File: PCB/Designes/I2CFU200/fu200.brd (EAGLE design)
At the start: 100 x 80 mm, 19 parts, among them IC2 LM358N, T1 2N3565, T2 2N3565, T3 2N3565, U1 ATMEGA328P-AU, X1 250-111, X3 250-706

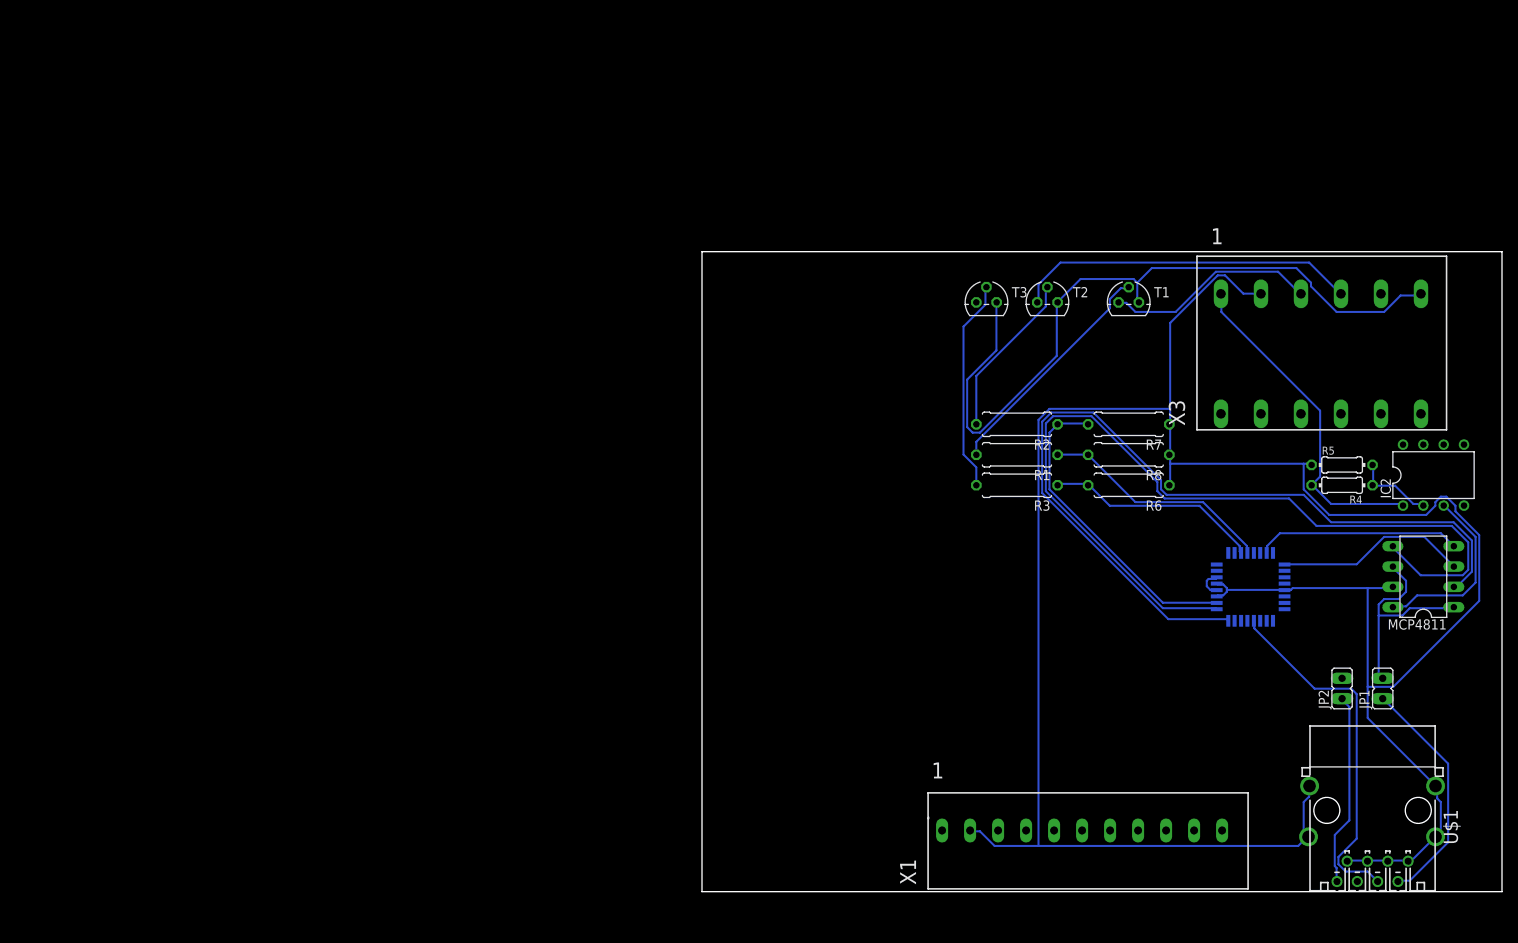
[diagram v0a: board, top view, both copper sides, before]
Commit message: ++
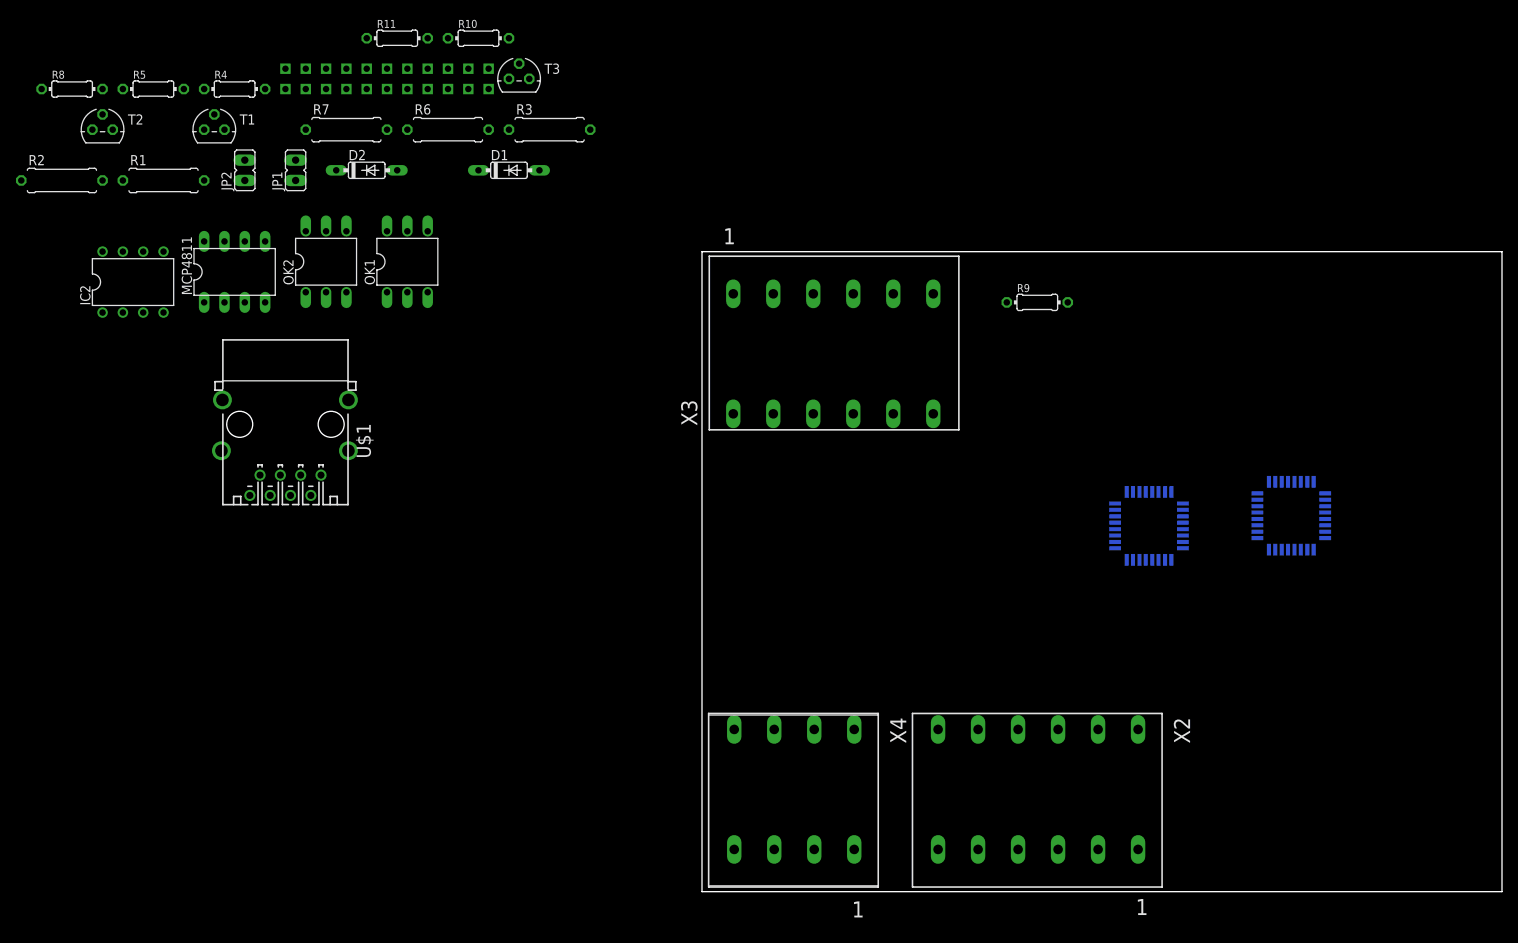
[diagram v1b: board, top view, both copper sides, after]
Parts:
- removed X1: 250-111, con-wago_250:P-250-111
- added D1, D2: 1N4148DO35-7, diode:DO35-7
- added OK1, OK2: CNY17, optocoupler:DIL06
- added R10, R11: 4,7kOhm, resistor:0204/7
- added R9: 1,2kOhm, resistor:0204/7
- added U$2: HUN_FU2, Btz:HUN_FU2
- added U2: ATMEGA328P-AU, Atmel-ATMEGA328P-AU:QFP80P900X900X120-32N
- added X2: 250-706, con-wago_250:P-250-706
- added X4: 250-704, con-wago_250:P-250-704
- R6, R7: value (none) -> R10K
- R8: value (none) -> 1,2kOhm; device resistor:0309/10 -> resistor:0204/7
- moved IC2 164.3 mm to (-71.1, 76.2)
- moved R5 155.8 mm to (-68.6, 100.3)
- moved MCP4811 153.4 mm to (-58.4, 77.5), turned to 0 degrees
- moved JP2 151.7 mm to (-57.1, 90.2)
- moved JP1 150.5 mm to (-50.8, 90.2)
- moved R4 147.0 mm to (-58.4, 100.3), turned to 0 degrees
- moved U$1 144.2 mm to (-52.1, 57.1)
- moved R8 139.8 mm to (-78.7, 100.3), turned to 0 degrees
- moved R2 123.2 mm to (-80.0, 88.9), turned to 0 degrees
- moved T2 120.1 mm to (-74.9, 95.2)
- moved T1 116.3 mm to (-61.0, 95.2)
- moved R1 112.1 mm to (-67.3, 88.9), turned to 0 degrees
- moved R7 104.5 mm to (-44.5, 95.2), turned to 0 degrees
- moved R6 96.0 mm to (-31.8, 95.2), turned to 0 degrees
- moved R3 73.4 mm to (-19.1, 95.2), turned to 0 degrees
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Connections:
- removed net DCM: T1.1, T2.1, T3.1, X3.L6.1
- removed net RST: T1.3, X3.L3.1
- new net +12V: X2.L1.2, X3.L1.1, X3.L3.1, X3.L5.1
- new net +5V: JP1.2, MCP4811.1, MCP4811.6, U1.4, U1.6, X3.L1.2, X3.L4.2, X3.L6.2, X4.L1.1, X4.L1.2
- new net DIR: X2.L5.2
- new net EN: X2.L4.2
- new net N$11: U$2.P$14
- new net N$17: U$2.P$1
- new net N$18: D1.C, OK1.1
- new net N$19: D2.C, OK2.1
- new net N$20: R9.2
- new net N$21: R10.1, R11.1
- new net N$22: OK2.5, R11.2
- new net N$23: R9.1, X3.L4.1
- new net N$24: R8.1, X3.L6.1
- new net N$25: OK1.5, R10.2
- new net N$3: U$2.P$5
- new net N$8: U$2.P$15
- new net N$9: U$2.P$6
- new net PUL: X2.L3.2
- new net RES: T1.1, X2.L3.1
- new net TEMP1: R6.2, U1.23, X3.L3.2
- new net TEMP2: R7.2, X3.L5.2
- new net VCC: U2.6
- new net VCC_2: U2.4
- net 0-10V: now also X2.L1.1; no longer X3.L1.1
- net AVCC: now also U2.18
- net FOR: now also T3.1, X2.L5.1; no longer T3.3, X3.L5.1
- net GND: now also D1.A, D2.A, OK1.2, OK1.4, OK2.2, OK2.4, T1.3, T2.3, T3.3, U2.3, U2.5, X2.L2.1, X2.L2.2, X2.L6.1, X2.L6.2, X3.L2.2, X4.L4.1, X4.L4.2; no longer R8.1, X1.L2
- net N$1: no longer R1.1, R8.2
- net N$12: no longer R7.2
- net N$13: now also R8.2; no longer JP1.2, MCP4811.1, MCP4811.6, U1.4, U1.6, X1.L1
- net N$15: no longer R6.2
- net N$32: no longer U1.32
- net N$37: no longer U1.1
- net REV: now also T2.1, X2.L4.1; no longer T2.3, X3.L4.1
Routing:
- net GND: track 302.8 -> 0.00 mm
- net N$37: track 111.0 -> 0.00 mm
- net N$32: track 107.3 -> 0.00 mm
- net DCM: track 93.0 -> 0.00 mm
- net N$6: track 45.2 -> 0.00 mm
- net REV: track 42.8 -> 0.00 mm
- net 0-10V: track 42.0 -> 0.00 mm
- net N$12: track 39.2 -> 0.00 mm
- net N$13: track 30.8 -> 0.00 mm
- net N$10: track 29.7 -> 0.00 mm
- net N$2: track 29.4 -> 0.00 mm
- net N$1: track 29.3 -> 0.00 mm
- net N$15: track 27.1 -> 0.00 mm
- net N$5: track 26.6 -> 0.00 mm
- net RST: track 26.5 -> 0.00 mm
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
